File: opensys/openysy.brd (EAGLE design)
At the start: 50 x 55 mm, 15 parts, among them M1 ARDUINO-NANO-3.0, M2 WIRELESS-NRF24L01, X1 USB

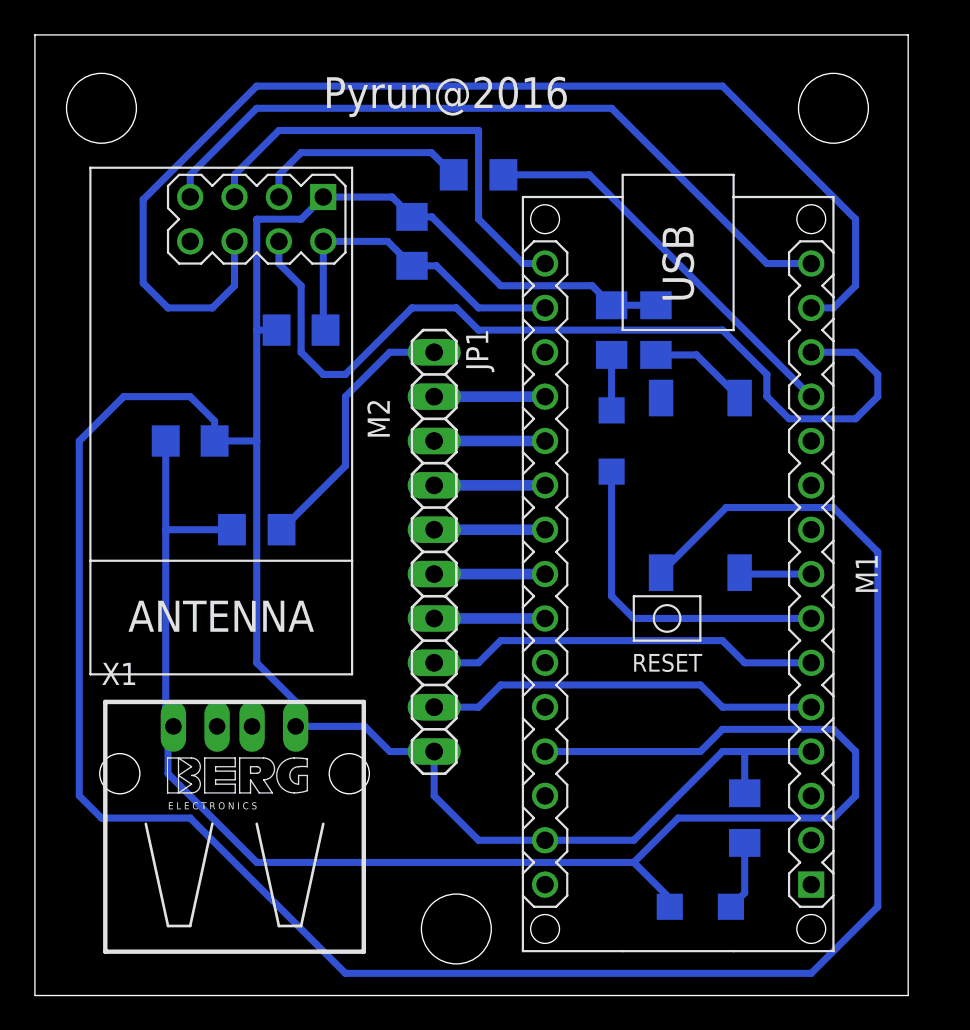
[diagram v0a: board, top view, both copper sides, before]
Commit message: smart home platine now v3
lets try it now
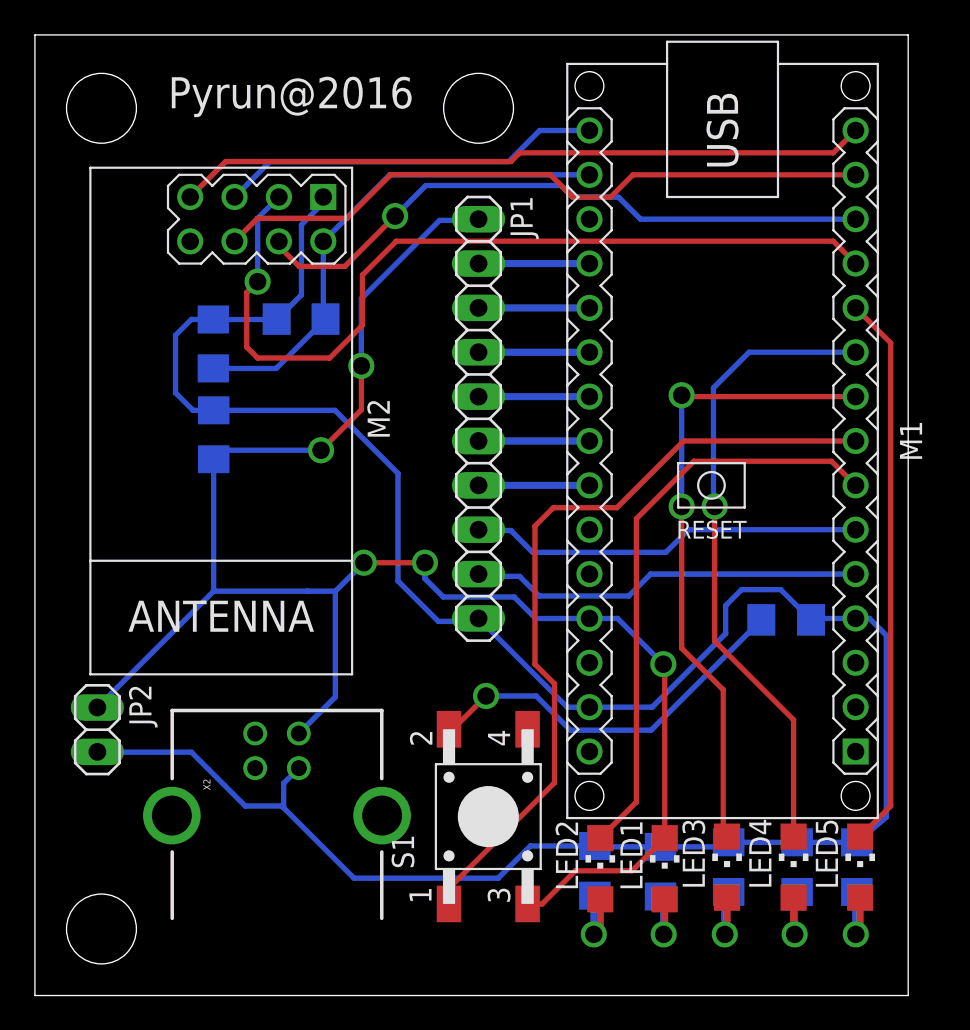
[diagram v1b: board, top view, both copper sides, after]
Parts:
- removed R3, R5: 0, rcl:R1206
- removed X1: USB, con-berg:PN87520
- added JP2: VCC, pinhead:1X02
- added LED3, LED4, LED5: 20mA, led:CHIPLED_1206
- added R6, R7, R8: 200, rcl:R1206
- added X2: USBPTH, usb:USB-B-PTH
- S1: value (none) -> S1
- moved R1 31.0 mm to (32.1, 7.14)
- moved LED2 24.5 mm to (32.4, 7.26), flipped to the top, turned to 0 degrees
- moved S1 22.5 mm to (26.0, 10.2), flipped to the top
- moved R2 18.2 mm to (43.0, 21.5), turned to 180 degrees
- moved C1 12.8 mm to (10.2, 37.3)
- moved JP1 8.03 mm to (25.4, 33.0)
- moved M1 8.03 mm to (39.4, 31.8)
- moved R4 5.71 mm to (35.8, 7.09)
- moved LED1 2.99 mm to (36.1, 7.26), flipped to the top, turned to 0 degrees
- moved C2 1.39 mm to (10.2, 32.1), turned to 270 degrees
- moved C3 0.62 mm to (15.2, 38.7)
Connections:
- net LED_0 renamed LED_TX
- removed net CE-TMP: M2.3, R3.2
- removed net LED_4: M1.J1.9
- removed net LED_5: M1.J1.10
- removed net LED_6: M1.J1.11
- removed net N$3: JP1.1, R5.1
- new net LED_1: LED3.C, M1.J1.9
- new net LED_2: LED4.C, M1.J1.10
- new net LED_3: LED5.C, M1.J1.11
- new net N$5: LED3.A, R6.1
- new net N$6: LED4.A, R7.1
- new net N$7: LED5.A, R8.1
- net CE: now also M2.3; no longer R3.1
- net GND: now also JP2.2, R6.2, R7.2, R8.2, X2.GND; no longer S1.3, X1.4
- net VCC: now also JP1.1, JP2.1, S1.3, X2.VBUS; no longer R5.2, X1.1
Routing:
- net GND: track 215.3 -> 137.4 mm
- net REG: track 4.13 -> 45.2 mm
- net LED_2: track 0.00 -> 36.6 mm, vias 0 -> 1
- net LED_1: track 0.00 -> 36.3 mm, vias 0 -> 2
- net LED_3: track 0.00 -> 31.8 mm
- net MOSI: track 67.2 -> 38.2 mm
- net CE: track 22.9 -> 49.5 mm, vias 0 -> 1
- net N$4: track 5.81 -> 22.1 mm, vias 0 -> 1
- net N$3: track 15.3 -> 0.00 mm
- net CSN: track 51.5 -> 36.5 mm, vias 0 -> 1
- net LED_TX: track 19.1 -> 33.6 mm
- net CE-TMP: track 12.3 -> 0.00 mm
- net +3V3: track 19.4 -> 28.9 mm
- net VCC: track 91.1 -> 99.5 mm, vias 0 -> 5
- net N$5: track 0.00 -> 4.88 mm, vias 0 -> 1
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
